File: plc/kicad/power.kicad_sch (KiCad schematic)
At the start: 73 parts, among them Q5 BSS138LT1G, Q6 CSD19537Q3, SW3 TSD003B08026A03, U15 TPS54560BDDAR, U16 TPS26630RGER, U17 TPS7A5201QRGRRQ1, U21 BZT52C3V3S

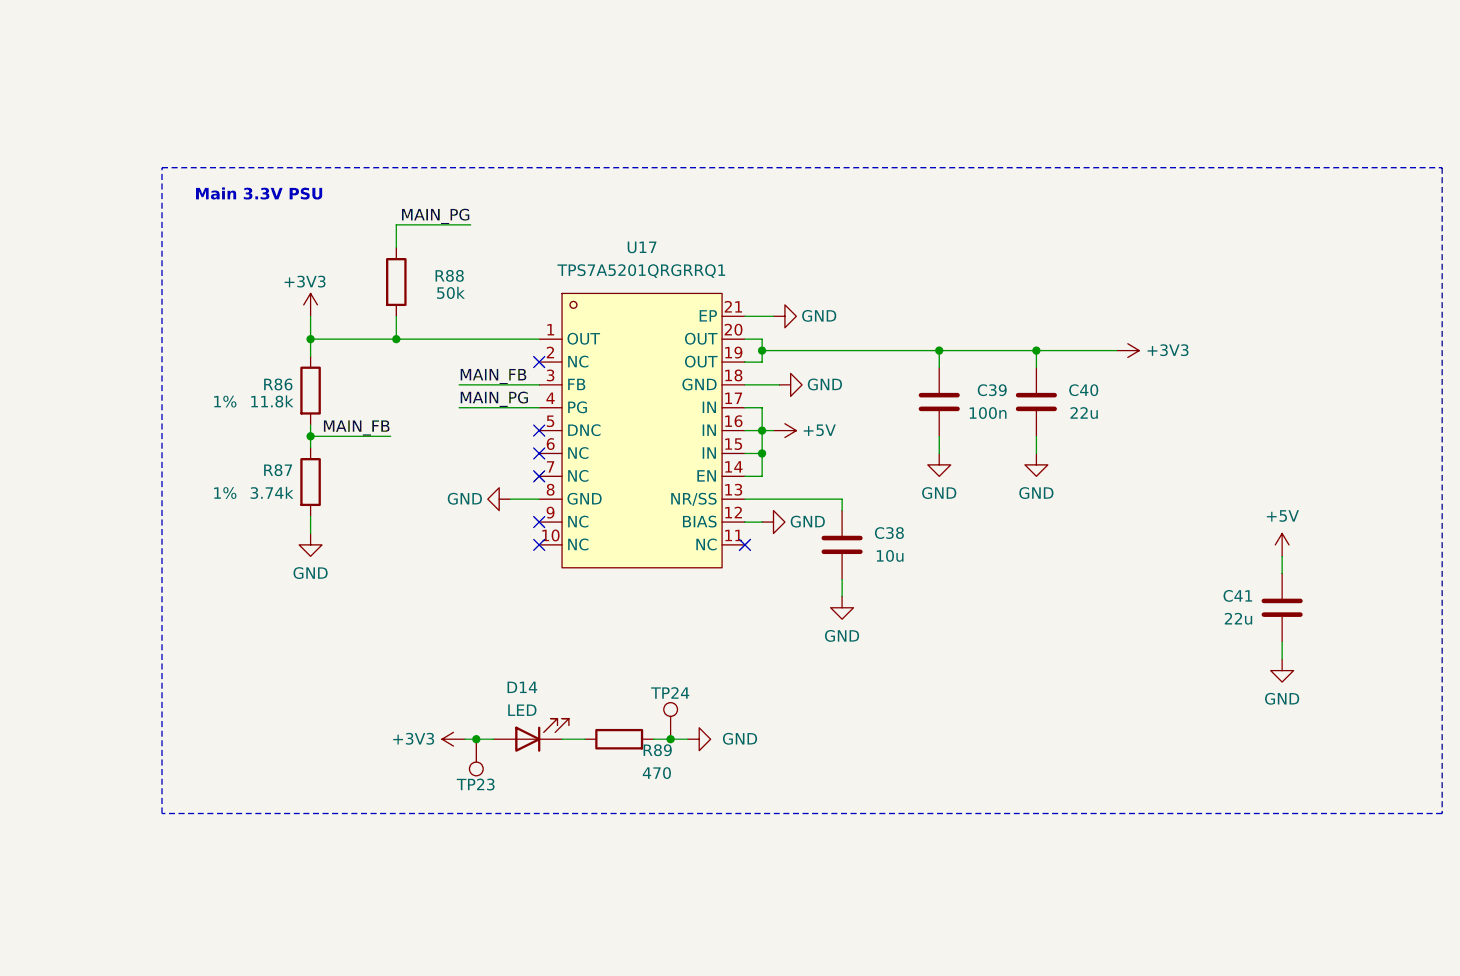
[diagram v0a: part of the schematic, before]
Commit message: Slight silkscreen & component adjustment
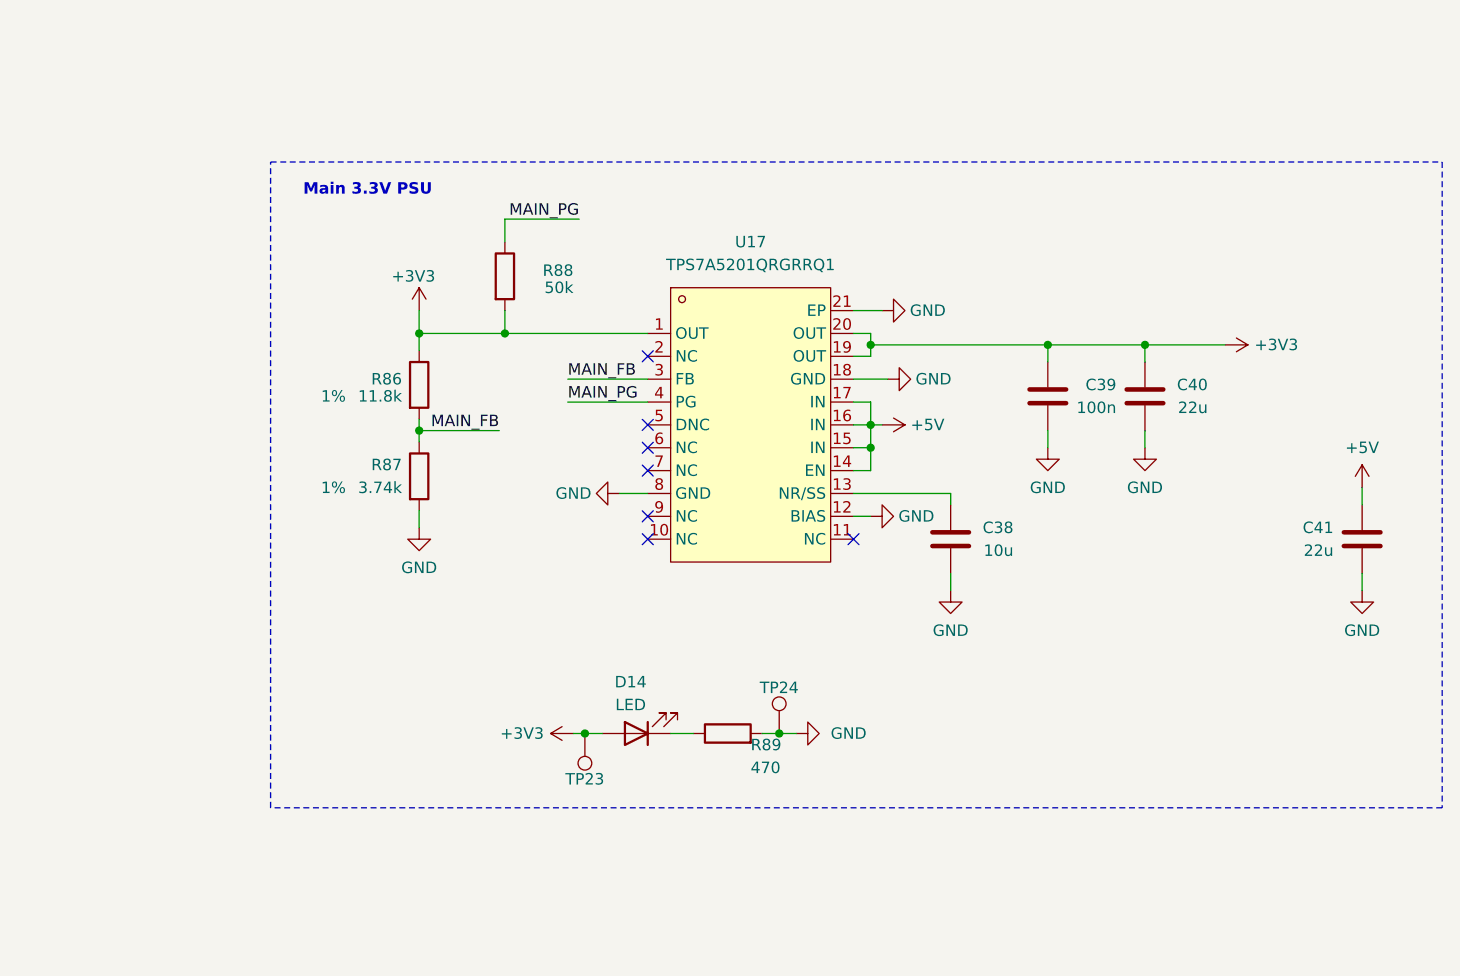
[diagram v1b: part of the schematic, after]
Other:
- moved on the sheet: C38, C39, C40, C41, D14, R86, R87, R88, R89, TP23, TP24, U17
